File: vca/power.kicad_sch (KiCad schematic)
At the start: 17 parts, among them U16 power_conn_16, U18 LM7805_TO220, U19 ZLDO1117G33TA

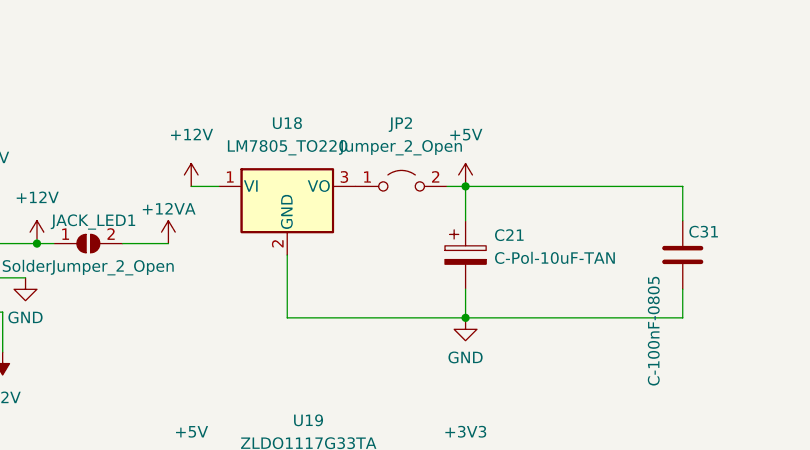
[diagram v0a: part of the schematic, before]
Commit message: working on the back panel power section
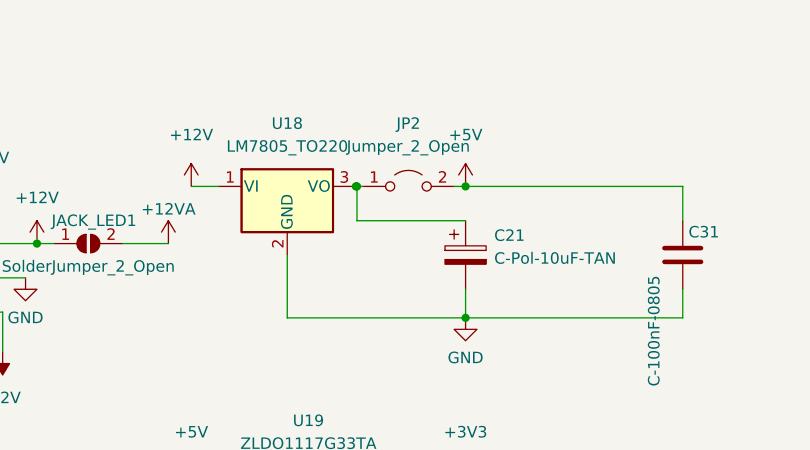
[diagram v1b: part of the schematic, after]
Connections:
- net +5V: no longer C21.1
- net at JP2.1 (A), U18.3 (VO): now also C21.1
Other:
- moved on the sheet: JP2
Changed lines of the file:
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@@
 (kicad_sch (version 20211123) (generator eeschema)
   (paper "A4")
+  (junction (at 97.79 28.575) (diameter 0) (color 0 0 0 0)
+  )
   (junction (at 109.855 43.18) (diameter 0) (color 0 0 0 0)
   )
@@
   )
   (junction (at 77.47 99.06) (diameter 0) (color 0 0 0 0)
+  )
+  (junction (at 97.663 28.575) (diameter 0) (color 0 0 0 0)
   )
   (junction (at 83.185 60.96) (diameter 0) (color 0 0 0 0)
@@
     (stroke (width 0) (type default) (color 0 0 0 0))
   )
+  (wire (pts (xy 98.425 28.575) (xy 97.79 28.575))
+    (stroke (width 0) (type default) (color 0 0 0 0))
+  )
   (wire (pts (xy 100.33 60.96) (xy 104.14 60.96))
     (stroke (width 0) (type default) (color 0 0 0 0))
@@
     (stroke (width 0) (type default) (color 0 0 0 0))
   )
-  (wire (pts (xy 107.823 28.575) (xy 109.855 28.575))
+  (wire (pts (xy 108.585 28.575) (xy 109.855 28.575))
     (stroke (width 0) (type default) (color 0 0 0 0))
   )
@@
     (stroke (width 0) (type default) (color 0 0 0 0))
   )
-  (wire (pts (xy 109.855 28.575) (xy 109.855 32.385))
+  (wire (pts (xy 109.855 32.385) (xy 97.79 32.385))
     (stroke (width 0) (type default) (color 0 0 0 0))
   )
@@
     (stroke (width 0) (type default) (color 0 0 0 0))
   )
+  (wire (pts (xy 97.79 28.575) (xy 97.79 32.385))
+    (stroke (width 0) (type default) (color 0 0 0 0))
+  )
   (wire (pts (xy 104.14 64.77) (xy 104.14 60.96))
     (stroke (width 0) (type default) (color 0 0 0 0))
   )
   (wire (pts (xy 71.755 90.17) (xy 71.755 88.9))
+    (stroke (width 0) (type default) (color 0 0 0 0))
+  )
+  (wire (pts (xy 97.79 28.575) (xy 97.663 28.575))
     (stroke (width 0) (type default) (color 0 0 0 0))
   )
@@
     (pin "2")
   )
-  (symbol (lib_id "Jumper:Jumper_2_Open") (at 102.743 28.575 0) (unit 1)
-    (in_bom yes) (on_board yes) (fields_autoplaced)
-    (property "Reference" "JP2" (id 0) (at 102.743 21.59 0))
-    (property "Value" "Jumper_2_Open" (id 1) (at 102.743 24.13 0))
-    (property "Footprint" "Jumper:SolderJumper-2_P1.3mm_Open_Pad1.0x1.5mm" (id 2) (at 102.743 28.575 0)
-      (effects (font (size 1.27 1.27)) hide)
-    )
-    (property "Datasheet" "~" (id 3) (at 102.743 28.575 0)
-      (effects (font (size 1.27 1.27)) hide)
-    )
+  (symbol (lib_id "Jumper:Jumper_2_Open") (at 103.505 28.575 0) (unit 1)
+    (in_bom yes) (on_board yes) (fields_autoplaced)
+    (property "Reference" "JP2" (id 0) (at 103.505 21.59 0))
+    (property "Value" "Jumper_2_Open" (id 1) (at 103.505 24.13 0))
+    (property "Footprint" "Jumper:SolderJumper-2_P1.3mm_Open_Pad1.0x1.5mm" (id 2) (at 103.505 28.575 0)
+      (effects (font (size 1.27 1.27)) hide)
+    )
+    (property "Datasheet" "~" (id 3) (at 103.505 28.575 0)
+      (effects (font (size 1.27 1.27)) hide)
+    )
